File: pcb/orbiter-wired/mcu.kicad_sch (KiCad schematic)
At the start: 24 parts, among them J4 AudioJack4, Q2 BSS138, SW30 SW_Push

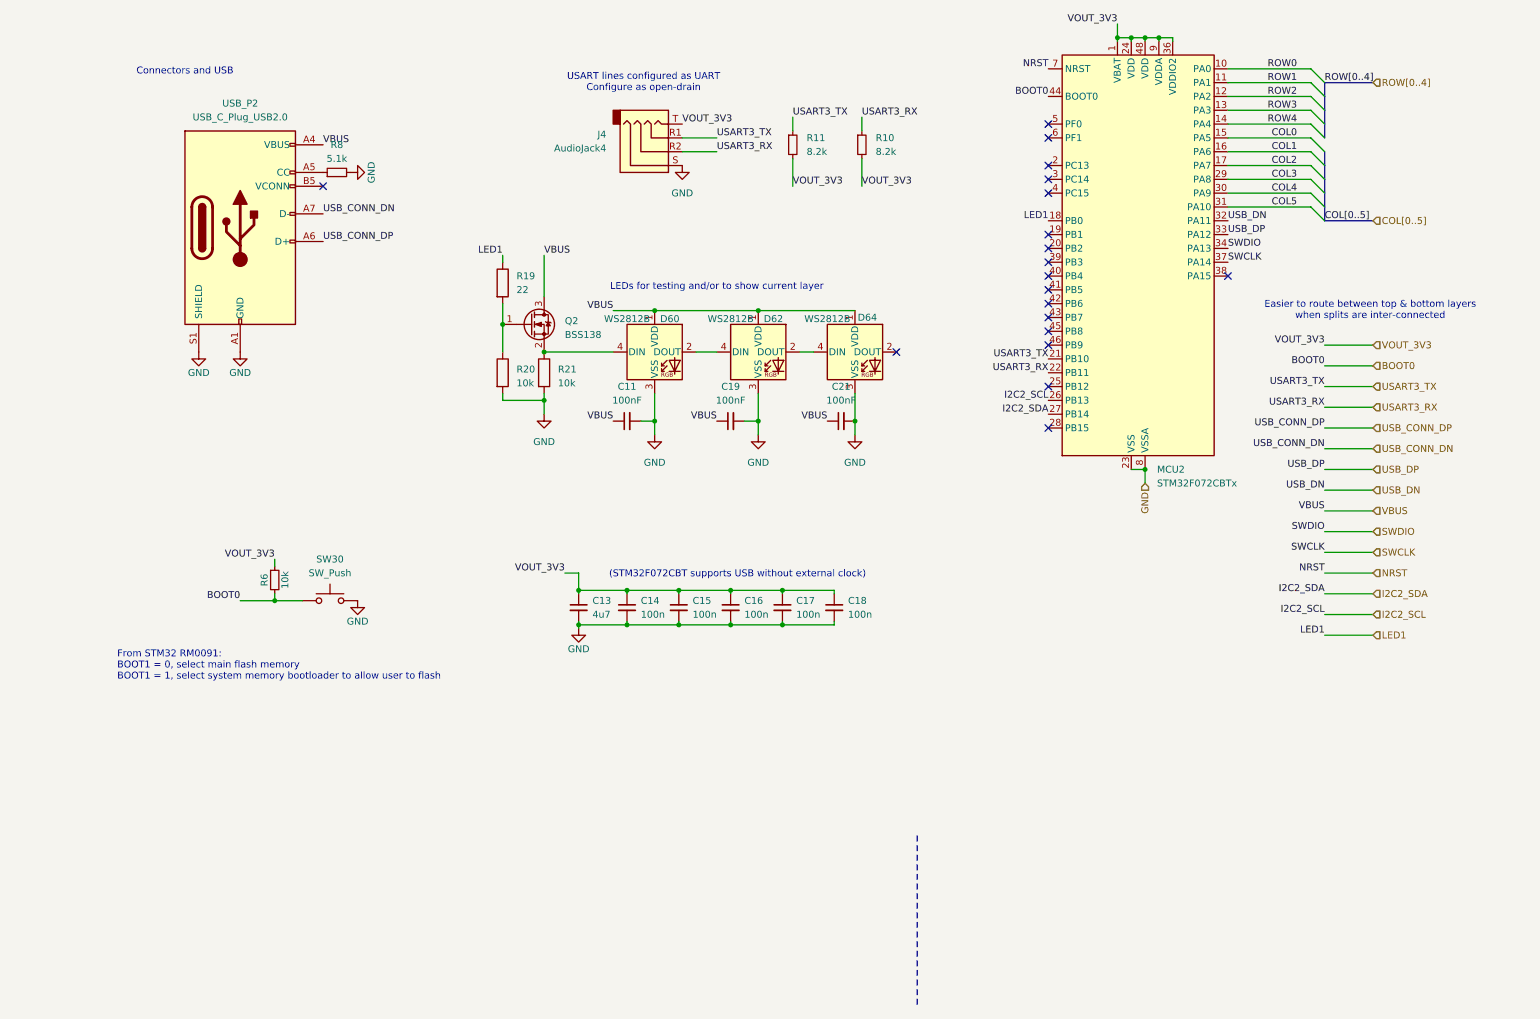
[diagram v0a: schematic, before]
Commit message: Add TODOs for fixes for next version
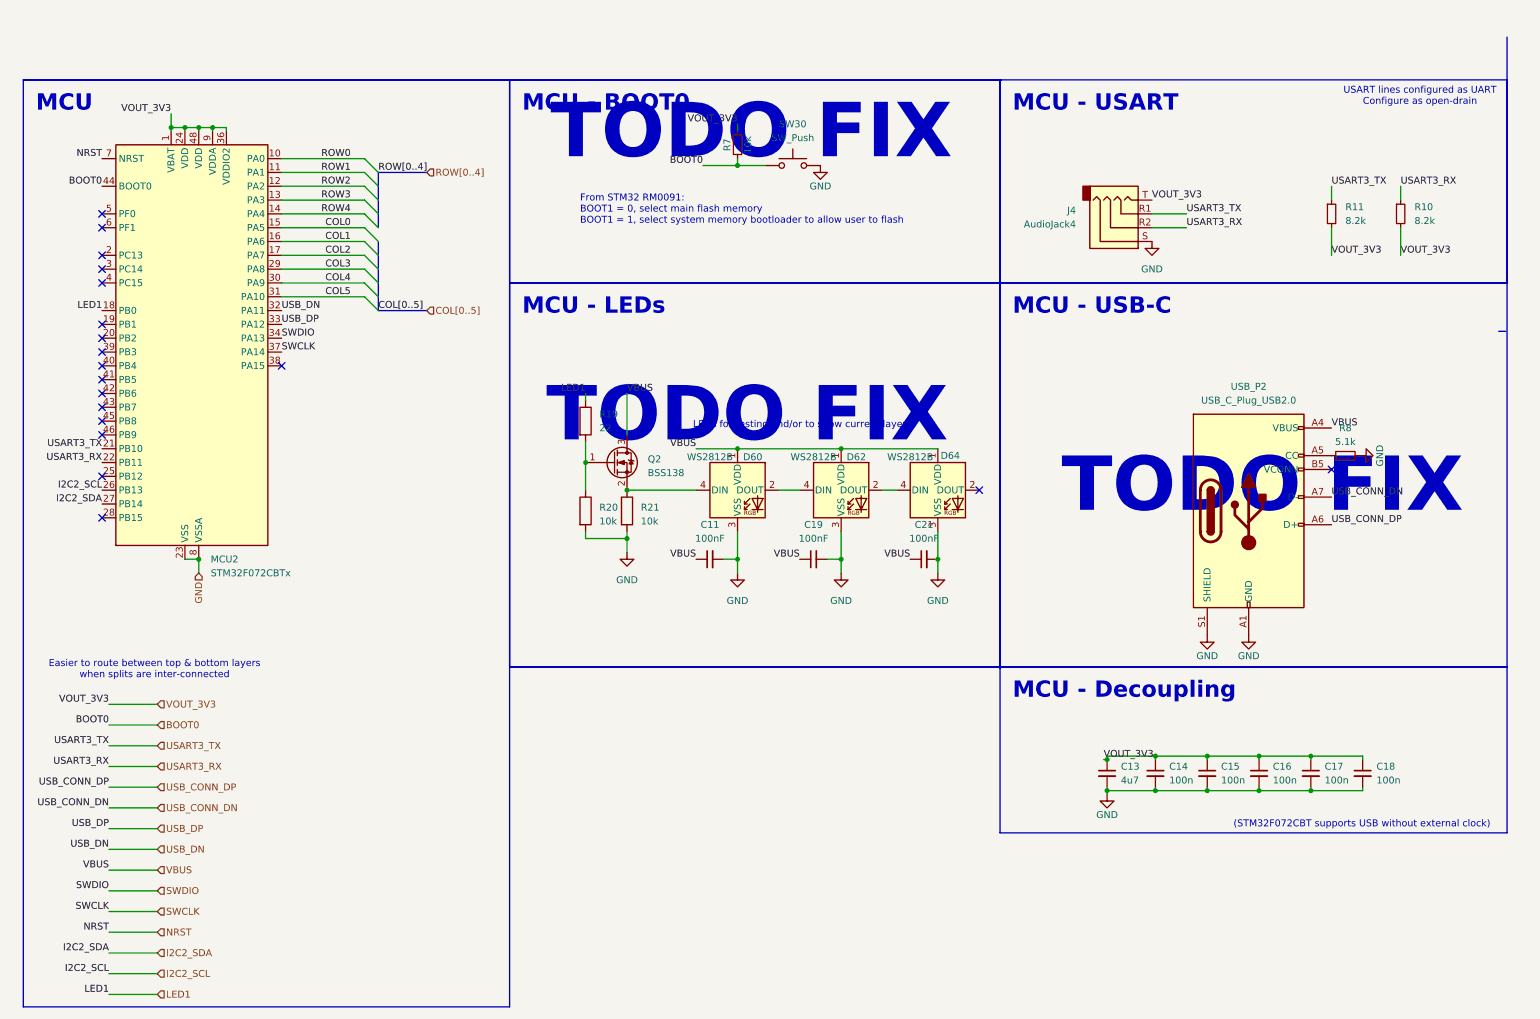
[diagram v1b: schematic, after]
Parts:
- renumbered R6 to R7
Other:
- note added: "TODO FIX"
- note removed: "Connectors and USB"
- moved on the sheet: C11, C13, C14, C15, C16, C17, C18, C19, C21, D60, D62, D64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
